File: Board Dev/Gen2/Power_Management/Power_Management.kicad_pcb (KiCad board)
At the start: 2 copper layers, 13 parts, among them IC1 MC33063AQDRQ1, K1 G5V-1 DC3, Q1 MCTL160N15Y-TP, Q2 MCTL160N15Y-TP, U1 ACS758ECB-200U-PFF-T

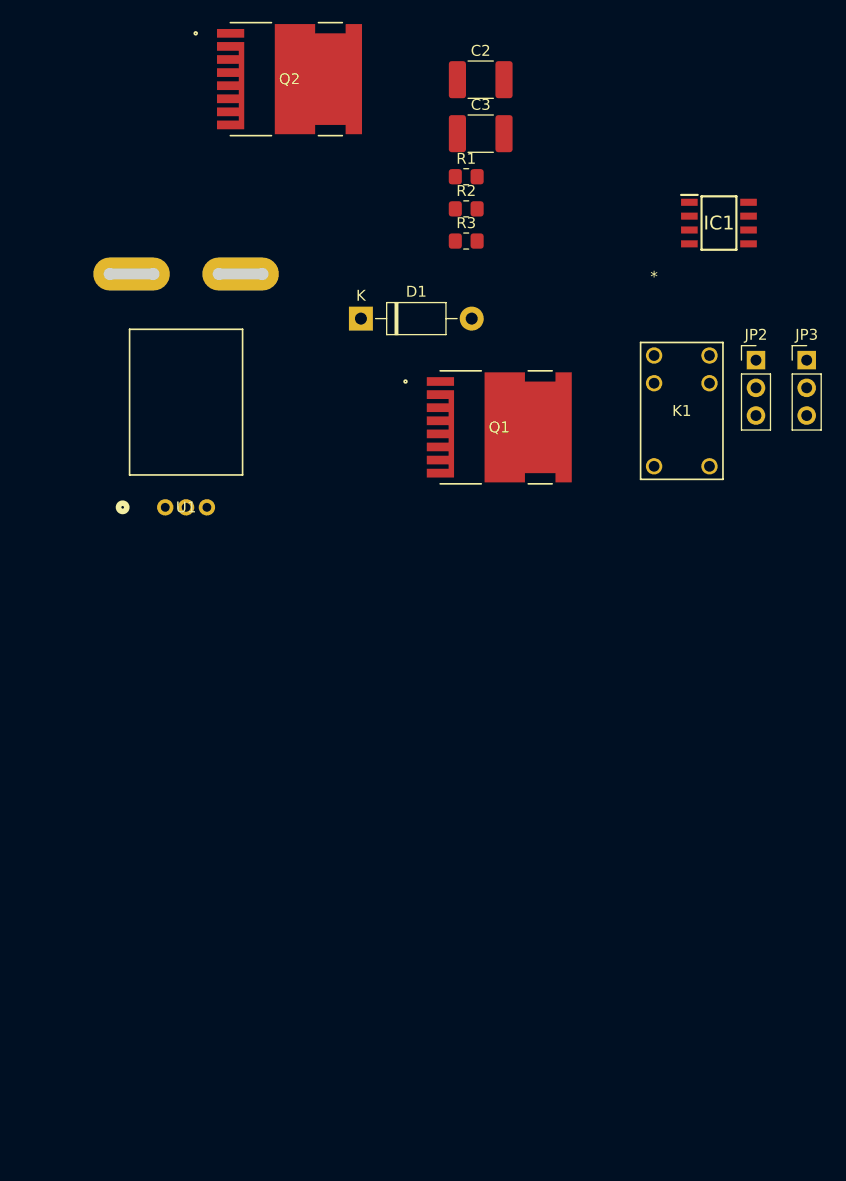
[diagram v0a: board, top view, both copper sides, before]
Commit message: done with management
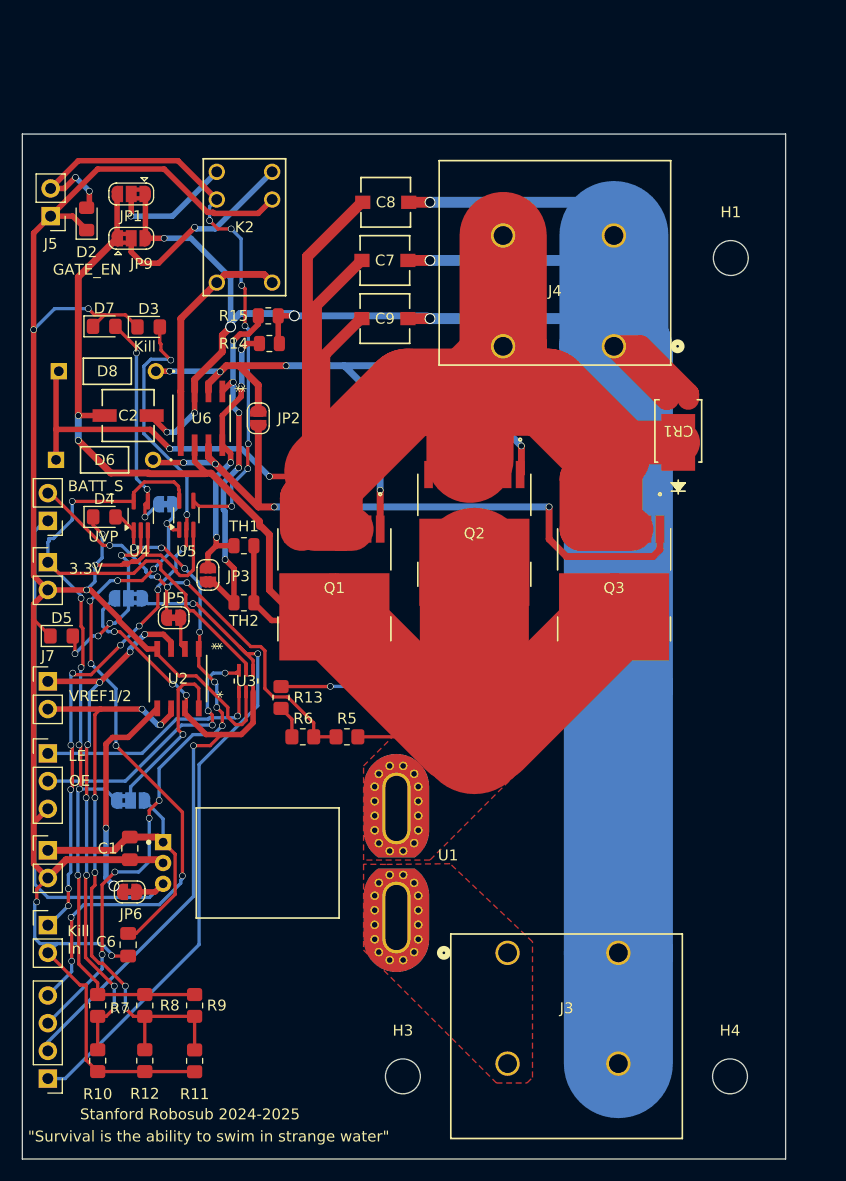
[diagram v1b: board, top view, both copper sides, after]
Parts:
- removed C3: 1uF, Capacitor_SMD:C_1812_4532Metric_Pad1.57x3.40mm_HandSolder
- removed D1: 1N5819, Diode_THT:D_DO-41_SOD81_P10.16mm_Horizontal
- removed IC1: MC33063AQDRQ1, Imported_Footprints:SOIC127P600X175-8N
- removed K1: G5V-1 DC3, Imported_Footprints:RELAY_G5V-1_OMR
- removed R1: 10k, Resistor_SMD:R_0805_2012Metric_Pad1.20x1.40mm_HandSolder
- removed R2: 10, Resistor_SMD:R_0805_2012Metric_Pad1.20x1.40mm_HandSolder
- removed R3: 100, Resistor_SMD:R_0805_2012Metric_Pad1.20x1.40mm_HandSolder
- added C1: 0.1u, Capacitor_SMD:C_0805_2012Metric_Pad1.18x1.45mm_HandSolder, F.Cu at (160.7, 155.8)
- added C6: 10uF, Capacitor_SMD:C_0805_2012Metric_Pad1.18x1.45mm_HandSolder, F.Cu at (160.5, 164.6)
- added C7: 1u, Imported_Footprints:U2-D_NCH, F.Cu at (184.1, 101.9)
- added C8: 1u, Imported_Footprints:U2-D_NCH, F.Cu at (184.2, 96.5)
- added C9: 1u, Imported_Footprints:U2-D_NCH, F.Cu at (184.1, 107.2)
- added CR1: SBRT15U50SP5-13, Imported_Footprints:POWERDI5_DIO, F.Cu at (211.0, 117.5)
- added D2: LED, LED_SMD:LED_0805_2012Metric_Pad1.15x1.40mm_HandSolder, F.Cu at (156.7, 98.0)
- added D3: LED, LED_SMD:LED_0805_2012Metric_Pad1.15x1.40mm_HandSolder, F.Cu at (162.4, 108.0)
- added D4: LED, LED_SMD:LED_0805_2012Metric_Pad1.15x1.40mm_HandSolder, F.Cu at (158.3, 125.4)
- added D5: LED, LED_SMD:LED_0805_2012Metric_Pad1.15x1.40mm_HandSolder, F.Cu at (154.4, 136.3)
- added D6: D_Zener, Imported_Footprints:1N5242B, F.Cu at (153.9, 120.1)
- added D7: LED, LED_SMD:LED_0805_2012Metric_Pad1.15x1.40mm_HandSolder, F.Cu at (158.3, 107.9)
- added D8: D_Zener, Imported_Footprints:1N5242B, F.Cu at (154.2, 112.0)
- added H1: MountingHole, MountingHole:MountingHole_3.2mm_M3, F.Cu at (215.8, 101.6)
- added H3: MountingHole, MountingHole:MountingHole_3.2mm_M3, F.Cu at (185.7, 176.7)
- added H4: MountingHole, MountingHole:MountingHole_3.2mm_M3, F.Cu at (215.7, 176.7)
- added J1: Conn_01x02_Pin, Connector_PinHeader_2.54mm:PinHeader_1x02_P2.54mm_Vertical, F.Cu at (153.2, 125.7)
- added J10: Conn_01x02_Pin, Connector_PinHeader_2.54mm:PinHeader_1x02_P2.54mm_Vertical, F.Cu at (153.2, 162.8)
- added J2: Conn_01x02_Pin, Connector_PinHeader_2.54mm:PinHeader_1x02_P2.54mm_Vertical, F.Cu at (153.2, 156.0)
- added J3: 1986660-2, Imported_Footprints:CONN2_1986660-2_TEC, F.Cu at (195.3, 165.4)
- added J4: 1986660-2, Imported_Footprints:CONN2_1986660-2_TEC, F.Cu at (205.1, 109.7)
- added J5: Conn_01x02_Pin, Connector_PinHeader_2.54mm:PinHeader_1x02_P2.54mm_Vertical, F.Cu at (153.4, 97.8)
- added J6: Conn_01x02_Pin, Connector_PinHeader_2.54mm:PinHeader_1x02_P2.54mm_Vertical, F.Cu at (153.2, 129.5)
- added J7: Conn_01x02_Pin, Connector_PinHeader_2.54mm:PinHeader_1x02_P2.54mm_Vertical, F.Cu at (153.2, 140.5)
- added J8: Conn_01x04_Pin, Connector_PinHeader_2.54mm:PinHeader_1x04_P2.54mm_Vertical, F.Cu at (153.2, 176.9)
- added J9: Conn_01x03_Pin, Connector_PinHeader_2.54mm:PinHeader_1x03_P2.54mm_Vertical, F.Cu at (153.2, 147.1)
- added JP1: SolderJumper_3_Bridged12, Jumper:SolderJumper-3_P1.3mm_Bridged2Bar12_RoundedPad1.0x1.5mm, F.Cu at (160.8, 95.8)
- added JP4: SolderJumper_3_Bridged12, Jumper:SolderJumper-3_P1.3mm_Bridged2Bar12_RoundedPad1.0x1.5mm, B.Cu at (160.8, 151.4)
- added JP5: SolderJumper_2_Bridged, Jumper:SolderJumper-2_P1.3mm_Bridged_RoundedPad1.0x1.5mm, F.Cu at (164.7, 134.6)
- added JP6: SolderJumper_2_Bridged, Jumper:SolderJumper-2_P1.3mm_Bridged_RoundedPad1.0x1.5mm, F.Cu at (160.7, 159.8)
- added JP7: SolderJumper_3_Bridged12, Jumper:SolderJumper-3_P1.3mm_Bridged2Bar12_RoundedPad1.0x1.5mm, B.Cu at (160.6, 132.8)
- added JP8: SolderJumper_2_Bridged, Jumper:SolderJumper-2_P1.3mm_Bridged_RoundedPad1.0x1.5mm, B.Cu at (164.0, 124.2)
- added JP9: SolderJumper_3_Bridged12, Jumper:SolderJumper-3_P1.3mm_Bridged2Bar12_RoundedPad1.0x1.5mm, F.Cu at (160.8, 99.8)
- added K2: G5V-1 DC3, Imported_Footprints:RELAY_G5V-1_OMR, F.Cu at (173.7, 103.9)
- added Q3: MCTL160N15Y-TP, Imported_Footprints:TOLL-8L_MCC, F.Cu at (205.1, 131.9)
- added R10: 200k, Resistor_SMD:R_0805_2012Metric_Pad1.20x1.40mm_HandSolder, F.Cu at (157.7, 175.2)
- added R11: ~, Resistor_SMD:R_0805_2012Metric_Pad1.20x1.40mm_HandSolder, F.Cu at (166.6, 175.3)
- added R12: ~, Resistor_SMD:R_0805_2012Metric_Pad1.20x1.40mm_HandSolder, F.Cu at (162.1, 175.2)
- added R13: 500k, Resistor_SMD:R_0805_2012Metric_Pad1.20x1.40mm_HandSolder, F.Cu at (174.5, 141.9)
- added R14: 100k, Resistor_SMD:R_0805_2012Metric, F.Cu at (173.5, 109.5)
- added R15: 100k, Resistor_SMD:R_0805_2012Metric, F.Cu at (173.4, 106.9)
- added R5: 100k, Resistor_SMD:R_0805_2012Metric_Pad1.20x1.40mm_HandSolder, F.Cu at (180.6, 145.5)
- added R6: 100k, Resistor_SMD:R_0805_2012Metric_Pad1.20x1.40mm_HandSolder, F.Cu at (176.5, 145.5)
- added R7: 150k, Resistor_SMD:R_0805_2012Metric_Pad1.20x1.40mm_HandSolder, F.Cu at (157.7, 170.2)
- added R8: ~, Resistor_SMD:R_0805_2012Metric_Pad1.20x1.40mm_HandSolder, F.Cu at (162.1, 170.2)
- added R9: ~, Resistor_SMD:R_0805_2012Metric_Pad1.20x1.40mm_HandSolder, F.Cu at (166.6, 170.2)
- added TH1: Thermistor_US, Resistor_SMD:R_0805_2012Metric, F.Cu at (171.1, 128.0)
- added TH2: Thermistor_US, Resistor_SMD:R_0805_2012Metric, F.Cu at (171.1, 133.3)
- added U2: LM393DT, Imported_Footprints:LM393DT, F.Cu at (165.1, 140.2)
- added U3: SN74LVC1G373DCKR, Imported_Footprints:SN74LVC, F.Cu at (171.3, 140.4)
- added U4: 74LVC1G08, Package_TO_SOT_SMD:SOT-353_SC-70-5_Handsoldering, F.Cu at (161.7, 125.3)
- added U5: 74LVC1G08, Package_TO_SOT_SMD:SOT-353_SC-70-5_Handsoldering, F.Cu at (165.9, 125.2)
- added U6: LTC1255CS8-PBF, Imported_Footprints:LTC1255, F.Cu at (167.3, 116.3)
- C2: value 1uF -> 10uF; footprint Capacitor_SMD:C_1812_4532Metric_Pad1.57x3.40mm_HandSolder -> Imported_Footprints:CAP_EEE-1CA100SR_PAN
- JP2, JP3: value Jumper_3_Bridged12 -> SolderJumper_2_Open; footprint Connector_PinHeader_2.54mm:PinHeader_1x03_P2.54mm_Vertical -> Jumper:SolderJumper-2_P1.3mm_Open_RoundedPad1.0x1.5mm
- U1: footprint Imported_Footprints:PFF_ACS758ECB-200U-PFF-T_ALM -> Imported_Footprints:Allegro_MicroSystems,_LLC-CB-5-PFF-0-0-MFG
- moved JP3 58.3 mm to (167.8, 130.7), turned to 90 degrees
- moved JP2 46.0 mm to (172.5, 116.3), turned to -90 degrees
- moved Q2 45.0 mm to (192.3, 126.9), turned to -90 degrees
- moved C2 44.7 mm to (160.5, 116.1)
- moved U1 33.9 mm to (173.3, 157.1), turned to -90 degrees
- moved Q1 21.1 mm to (179.4, 131.9), turned to -90 degrees
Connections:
- C2 pad 1: Sense(+) -> /FETs/+Batt
- C2 pad 2: Net-(U2-OUT) -> /Battery_input/-Batt
- JP2 pad 1: +25V -> /FETs/GATE1_DRIVE
- JP2 pad 2: Net-(JP2-C) -> /FETs/GATE2_DRIVE
- JP3 pad 1: -BATT -> Net-(JP3-A)
- Q1 pad 1: GATE_DRIVE -> /FETs/GATE1_DRIVE
- Q1 pad 2: -BATT -> /FETs/V_THRUST
- Q1 pad 3: -BATT -> /FETs/V_THRUST
- Q1 pad 4: -BATT -> /FETs/V_THRUST
- Q1 pad 5: -BATT -> /FETs/V_THRUST
- Q1 pad 6: -BATT -> /FETs/V_THRUST
- Q1 pad 7: -BATT -> /FETs/V_THRUST
- Q1 pad 8: -BATT -> /FETs/V_THRUST
- Q1 pad 9: +BATT -> /FETs/+Batt
- Q2 pad 1: GATE_DRIVE -> /FETs/GATE1_DRIVE
- Q2 pad 2: -BATT -> /FETs/V_THRUST
- Q2 pad 3: -BATT -> /FETs/V_THRUST
- Q2 pad 4: -BATT -> /FETs/V_THRUST
- Q2 pad 5: -BATT -> /FETs/V_THRUST
- Q2 pad 6: -BATT -> /FETs/V_THRUST
- Q2 pad 7: -BATT -> /FETs/V_THRUST
- Q2 pad 8: -BATT -> /FETs/V_THRUST
- Q2 pad 9: +BATT -> /FETs/+Batt
- U1 pad 3: /VSENSE_ANALOG -> /OCP_UVP_detect/ISENSE_ANALOG
- U1 pad 4: +BATT_HALL -> /Battery_input/+BATT_HALL
- U1 pad 5: +BATT -> /FETs/+Batt
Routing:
- net /Battery_input/-Batt: track 0.00 -> 238.5 mm, vias 0 -> 9
- net GND: track 0.00 -> 214.0 mm, vias 0 -> 7
- net /FETs/V_THRUST: track 0.00 -> 203.8 mm, vias 0 -> 2
- net /FETs/+Batt: track 0.00 -> 133.8 mm, vias 0 -> 2
- net +3.3V: track 0.00 -> 98.5 mm, vias 0 -> 6
- net /FET_control_logic/Kill_Switch: track 0.00 -> 65.7 mm, vias 0 -> 11
- net Net-(J8-Pin_4): track 0.00 -> 64.1 mm, vias 0 -> 9
- net /FET_control_logic/OCP_LATCH: track 0.00 -> 63.2 mm, vias 0 -> 2
- net /FETs/GATE2_DRIVE: track 0.00 -> 63.1 mm, vias 0 -> 4
- net /FETs/GATE1_DRIVE: track 0.00 -> 63.0 mm, vias 0 -> 5
- net /FET_control_logic/OCP_COMP: track 0.00 -> 61.4 mm, vias 0 -> 4
- net /FET_control_logic/UVP_COMP: track 0.00 -> 61.4 mm, vias 0 -> 11
- net /FET_control_logic/3.3V_GATE_EN: track 0.00 -> 58.5 mm, vias 0 -> 9
- net VREF2: track 0.00 -> 54.9 mm, vias 0 -> 6
- net VREF1: track 0.00 -> 50.7 mm, vias 0 -> 8
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- added copper zone on F.Cu, net /Battery_input/+BATT_HALL
- added copper zone on F.Cu, net /FETs/+Batt
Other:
- board outline added: 70 x 94 mm
- board text added: "3.3V"
- board text added: "BATT_S"
- board text added: "GATE_EN"
- board text added: "Kill"
- board text added: "Kill In"
- board text added: "LE"
- board text added: "OE"
- board text added: "Stanford Robosub 2024-2025"
- board text added: "UVP"
- board text added: "VREF1/2"
- board text added: "{dblquote}Survival is the ability to swim in strange water{dblquote}"
